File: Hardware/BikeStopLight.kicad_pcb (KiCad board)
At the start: 2 copper layers, 63 parts, among them J1 ST-Link, J2 PWR, J3 BAT, J4 Conn_01x01, J5 Conn_01x01, J6 Conn_01x08, Q1 NTD4909N, U1 MCP1703A-3302_SOT23, U2 STM32L052K8Tx, U3 RFM95W-868S2, Y1 ABS07-120-32.768KHZ-T

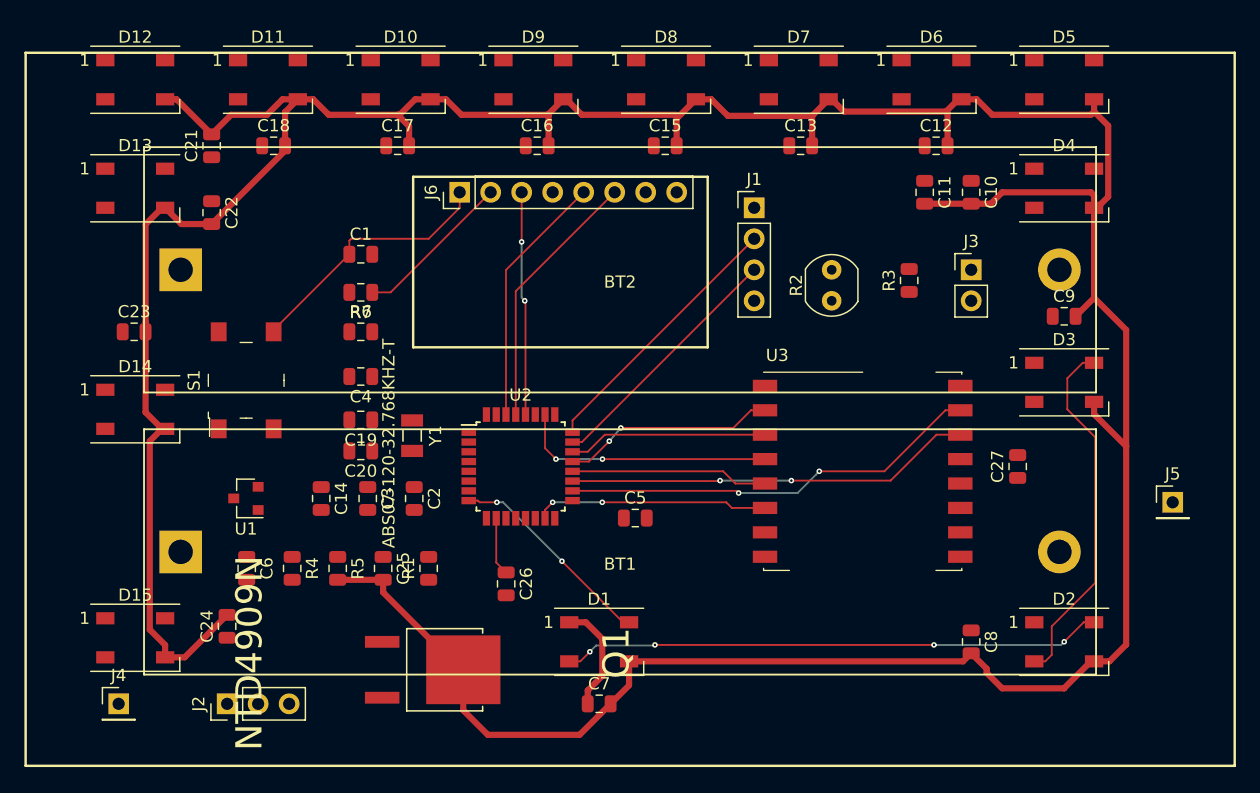
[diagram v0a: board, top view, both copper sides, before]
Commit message: WIP - Routed
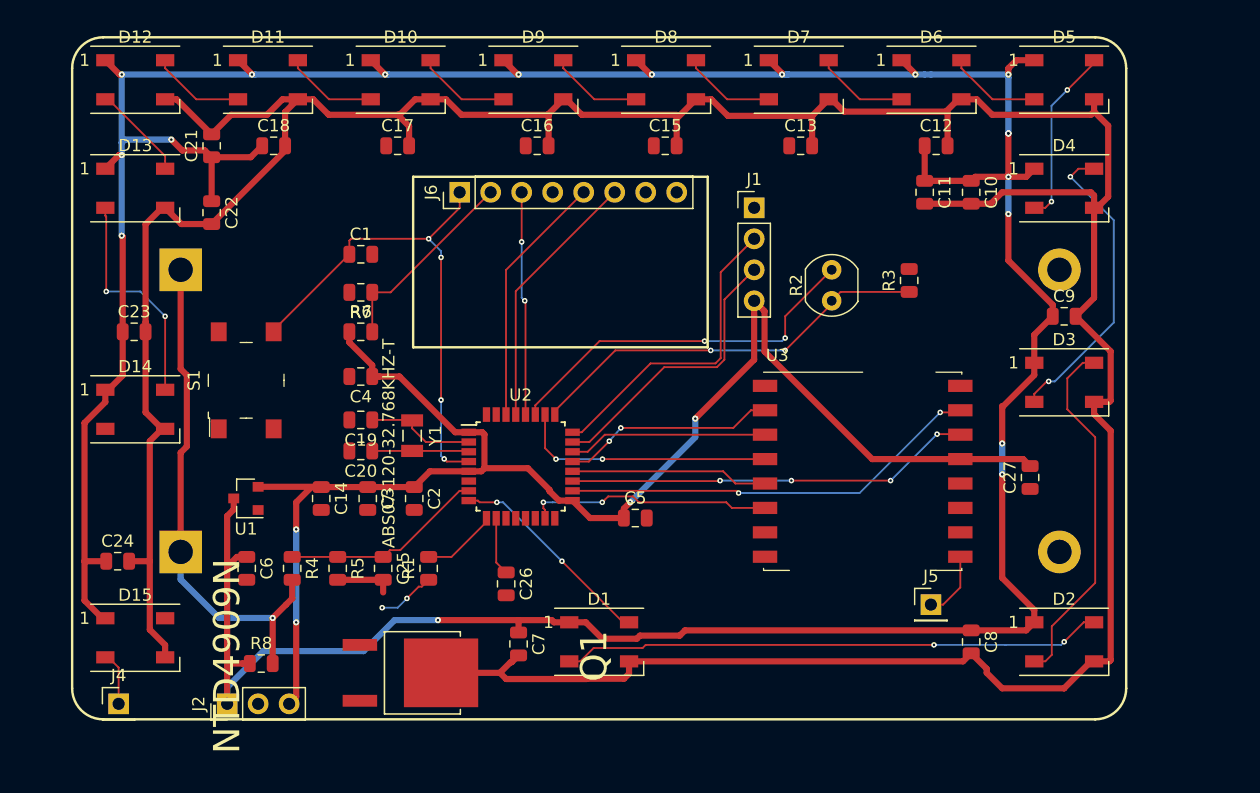
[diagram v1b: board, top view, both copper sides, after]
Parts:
- removed J3: BAT, Connector_PinHeader_2.54mm:PinHeader_1x02_P2.54mm_Vertical
- added R8: 0 Ohm, Resistor_SMD:R_0805_2012Metric, F.Cu at (44.7, 169.4)
- BT1, BT2: moved to B.Cu
- moved J5 21.5 mm to (99.6, 164.6)
- moved C24 10.4 mm to (32.9, 161.0), turned to 0 degrees
- moved C7 8.23 mm to (65.8, 167.8), turned to 270 degrees
- moved Q1 1.84 mm to (56.9, 170.2)
- moved C27 1.36 mm to (107.7, 154.2)
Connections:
- C27 pad 2: VCC -> +3V3
- U3 pad 13: VCC -> +3V3
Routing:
- net VCC: track 9.09 -> 308.7 mm, vias 0 -> 18
- net +3V3: track 0.00 -> 122.4 mm, vias 0 -> 4
- net +BATT: track 0.00 -> 42.2 mm, vias 0 -> 1
- net /LDR_OUT: track 0.00 -> 33.5 mm, vias 0 -> 2
- net /LDR_PWR: track 0.00 -> 30.7 mm, vias 0 -> 2
- net Net-(D3-Pad2): track 0.00 -> 25.2 mm, vias 0 -> 2
- net GNDPWR: track 309.2 -> 288.1 mm
- net /NRST: track 21.5 -> 42.1 mm, vias 0 -> 4
- net Net-(D13-Pad2): track 0.00 -> 18.6 mm, vias 0 -> 2
- net /VBat_Scale: track 0.00 -> 16.7 mm
- net Net-(D4-Pad2): track 0.00 -> 14.6 mm, vias 0 -> 2
- net Net-(C19-Pad1): track 0.00 -> 9.04 mm
- net Net-(C20-Pad1): track 0.00 -> 7.94 mm
- net Net-(D12-Pad2): track 0.00 -> 7.87 mm
- net /LED_D5_DOUT: track 0.00 -> 7.68 mm
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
